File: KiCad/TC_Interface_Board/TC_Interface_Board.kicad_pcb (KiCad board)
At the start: 2 copper layers, 30 parts, among them J10 Conn_01x05, J11 Conn_01x05, J1_24V_ROW1 Conn_01x04, J1_CN1_24V1 Conn_01x03, J2_CN2_9V_Main1 Conn_01x02, J3_CN3_9V_Main1 Conn_01x02, J4 Conn_01x05, J5 Conn_01x05, J6 Conn_01x05, J7 Conn_01x05, J8 Conn_01x05, J9 Conn_01x05, Q1 DTC143E, Q2 DTC143E, U1 MC34063AP

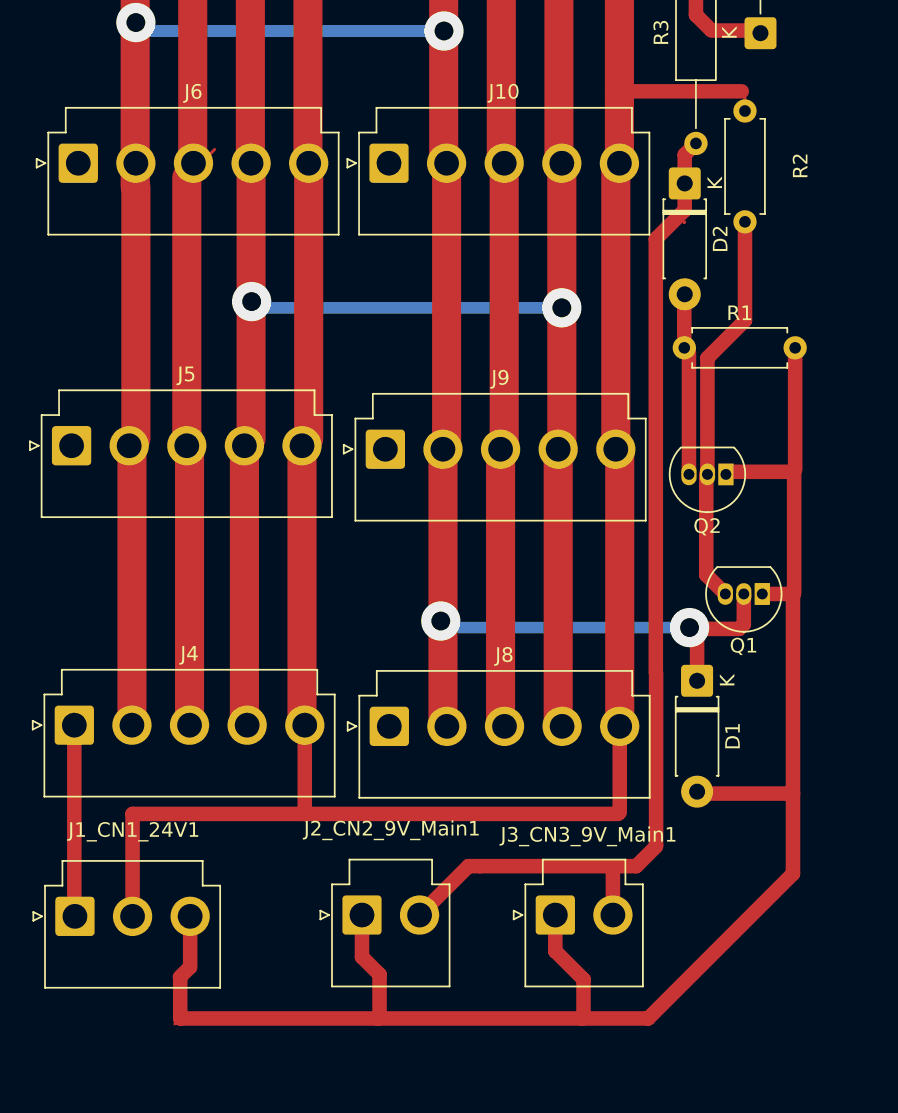
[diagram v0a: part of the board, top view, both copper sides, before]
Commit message: UPDATE
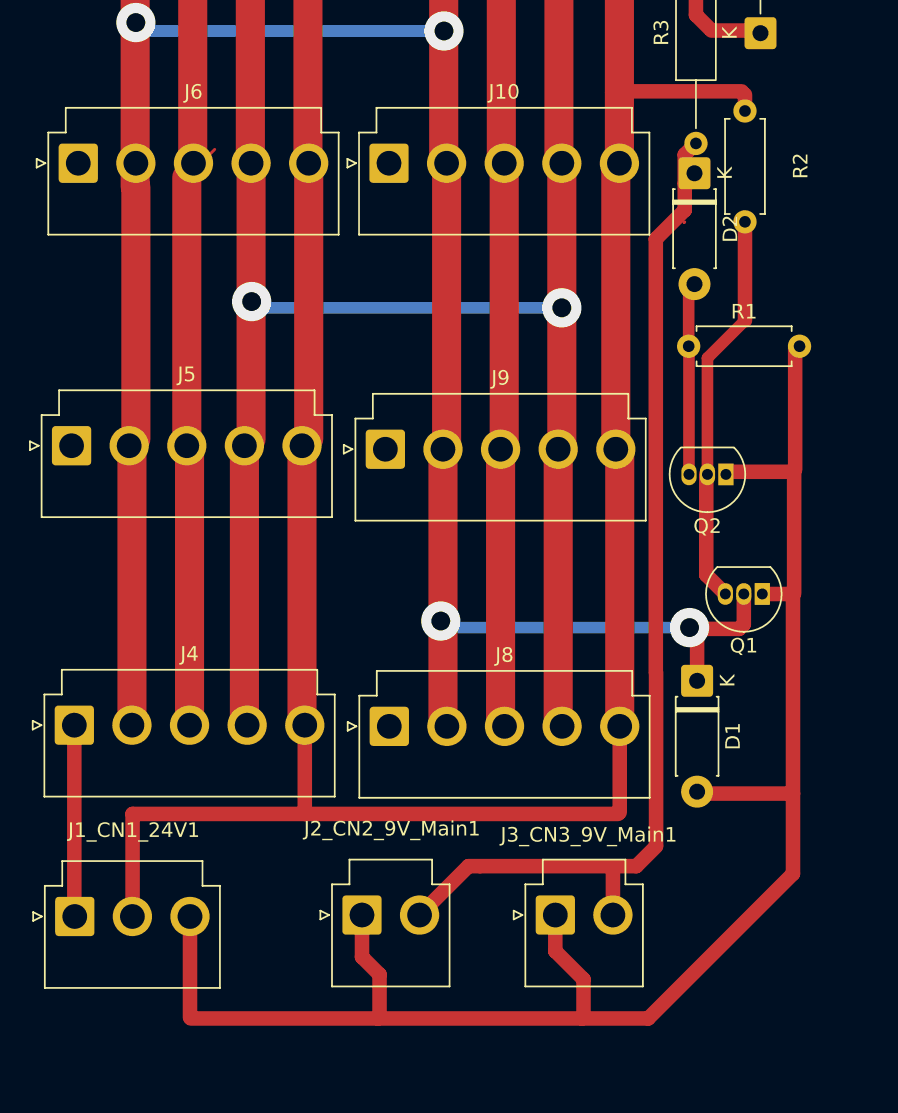
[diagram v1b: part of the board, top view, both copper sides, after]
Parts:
- moved D2 0.97 mm to (166.3, 89.9)
- moved R1 0.32 mm to (165.9, 101.8)
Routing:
- net Net-(D1-A): track 121.5 -> 119.9 mm
- net Net-(D2-A): track 12.5 -> 13.3 mm
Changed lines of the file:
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@@
 	(footprint "Resistor_THT:R_Axial_DIN0207_L6.3mm_D2.5mm_P7.62mm_Horizontal"
 		(layer "F.Cu")
-		(at 165.64 101.92)
+		(at 165.94 101.81)
 		(descr "Resistor, Axial_DIN0207 series, Axial, Horizontal, pin pitch=7.62mm, 0.25W = 1/4W, length*diameter=6.3*2.5mm^2, http://cdn-reichelt.de/documents/datenblatt/B400/1_4W%23YAG.pdf")
 		(tags "Resistor Axial_DIN0207 series Axial Horizontal pin pitch 7.62mm 0.25W = 1/4W length 6.3mm diameter 2.5mm")
@@
 	(footprint "Diode_THT:D_DO-41_SOD81_P7.62mm_Horizontal"
 		(layer "F.Cu")
-		(at 165.67 90.62 -90)
+		(at 166.34 89.92 -90)
 		(descr "Diode, DO-41_SOD81 series, Axial, Horizontal, pin pitch=7.62mm, length*diameter=5.2*2.7mm^2, https://www.diodes.com/assets/Package-Files/DO-41-Plastic.pdf")
 		(tags "Diode DO-41_SOD81 series Axial Horizontal pin pitch 7.62mm  length 5.2mm diameter 2.7mm")
@@
 	(footprint "Connector_JST:JST_VH_B3P-VH-B_1x03_P3.96mm_Vertical"
 		(layer "F.Cu")
-		(at 123.7525 141)
+		(at 123.74 141.01)
 		(descr "JST VH PBT series connector, B3P-VH-B (http://www.jst-mfg.com/product/pdf/eng/eVH.pdf), generated with kicad-footprint-generator")
 		(tags "connector JST VH vertical")
@@
 		(start 165.96 110.62)
 		(end 165.96 102.24)
-		(width 1)
+		(width 0.8)
 		(layer "F.Cu")
 		(net 2)
 	)
 	(segment
-		(start 165.64 101.92)
-		(end 165.64 98.27)
-		(width 1)
+		(start 165.94 97.94)
+		(end 166.34 97.54)
+		(width 0.2)
 		(layer "F.Cu")
 		(net 2)
@@
 	)
 	(segment
+		(start 165.94 101.81)
+		(end 165.94 97.94)
+		(width 0.8)
+		(layer "F.Cu")
+		(net 2)
+	)
+	(segment
 		(start 162.43 58.71)
 		(end 162.43 60.646428)
@@
 	)
 	(segment
-		(start 130.966428 145.18)
-		(end 131.626428 144.52)
-		(width 1)
-		(layer "F.Cu")
-		(net 8)
-	)
-	(segment
 		(start 168.68 110.44)
 		(end 168.5 110.62)
@@
 	)
 	(segment
-		(start 130.99 148.02)
-		(end 144.58 148.02)
-		(width 1)
-		(layer "F.Cu")
-		(net 8)
-	)
-	(segment
 		(start 173.16 118.84)
 		(end 173.19 118.81)
@@
 	)
 	(segment
-		(start 131.656428 144.52)
-		(end 131.6725 144.503928)
-		(width 0.2)
-		(layer "F.Cu")
-		(net 8)
-	)
-	(segment
 		(start 158.71 145.33)
 		(end 158.71 147.91)
@@
 	)
 	(segment
+		(start 131.72 148.02)
+		(end 144.58 148.02)
+		(width 1)
+		(layer "F.Cu")
+		(net 8)
+	)
+	(segment
 		(start 144.58 148.02)
 		(end 158.6 148.02)
@@
 	)
 	(segment
-		(start 130.99 145.203572)
-		(end 130.966428 145.18)
-		(width 0.2)
+		(start 173.11 132.56)
+		(end 173.11 118.96)
+		(width 1)
 		(layer "F.Cu")
 		(net 8)
 	)
 	(segment
-		(start 173.11 132.56)
-		(end 173.11 118.96)
-		(width 1)
+		(start 131.72 148.02)
+		(end 131.66 147.96)
+		(width 0.2)
 		(layer "F.Cu")
 		(net 8)
@@
 	)
 	(segment
-		(start 131.6725 144.503928)
-		(end 131.6725 141)
-		(width 1)
-		(layer "F.Cu")
-		(net 8)
-	)
-	(segment
 		(start 173.26 110.29)
 		(end 173.26 101.92)
@@
 	)
 	(segment
-		(start 131.626428 144.52)
-		(end 131.656428 144.52)
-		(width 0.2)
-		(layer "F.Cu")
-		(net 8)
-	)
-	(segment
 		(start 143.4825 143.7925)
 		(end 144.69 145)
@@
 	)
 	(segment
-		(start 130.61 148.4)
-		(end 130.99 148.02)
-		(width 0.2)
+		(start 131.66 147.96)
+		(end 131.66 141.01)
+		(width 1)
 		(layer "F.Cu")
 		(net 8)
@@
 	)
 	(segment
-		(start 130.99 148.02)
-		(end 130.99 145.203572)
-		(width 1)
-		(layer "F.Cu")
-		(net 8)
-	)
-	(segment
 		(start 167.15 117.53)
 		(end 167.15 110.62)
@@
 		(start 167.23 102.62)
 		(end 169.81 100.04)
-		(width 1)
+		(width 0.8)
 		(layer "F.Cu")
 		(net 9)
@@
 		(start 167.23 110.62)
 		(end 167.23 102.62)
-		(width 1)
+		(width 0.8)
 		(layer "F.Cu")
 		(net 9)
@@
 		(start 169.81 85.64)
 		(end 169.81 84.51)
-		(width 0.2)
+		(width 1)
 		(layer "F.Cu")
 		(net 16)

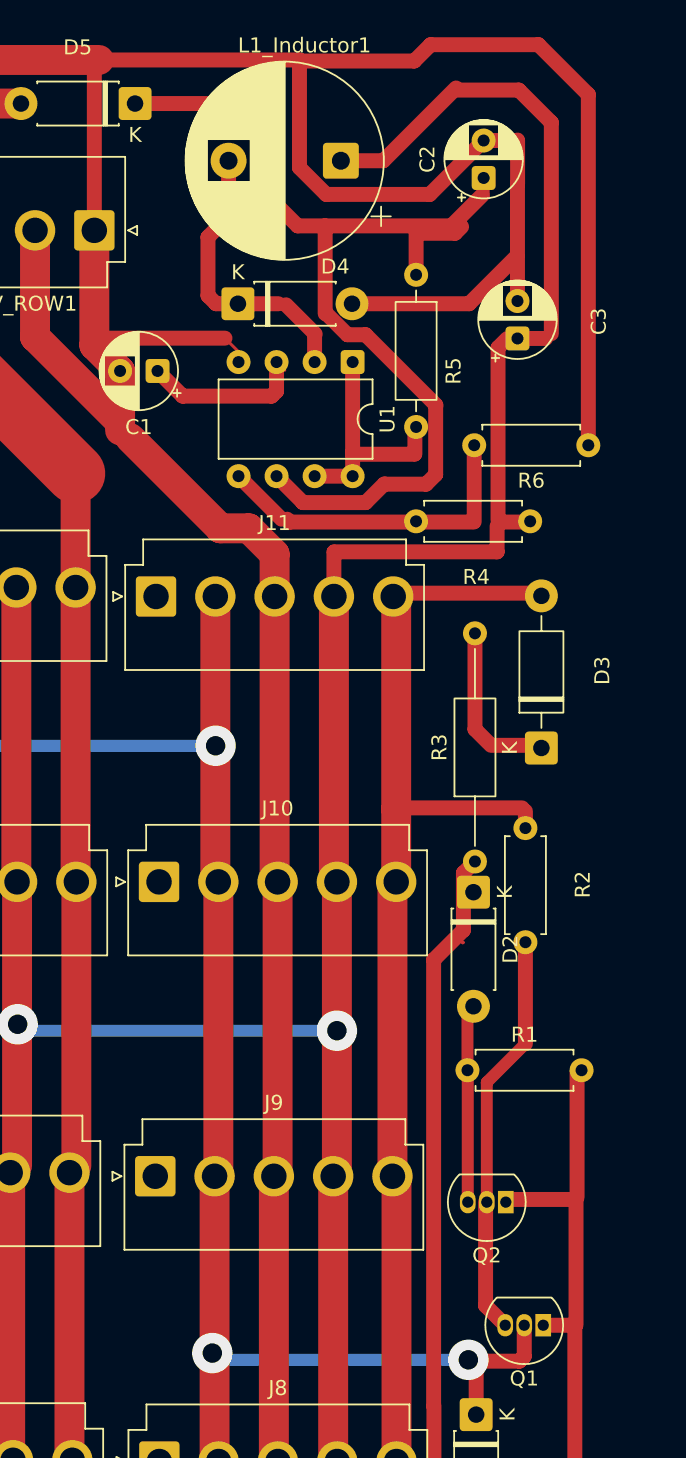
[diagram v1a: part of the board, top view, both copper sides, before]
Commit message: UPDATE
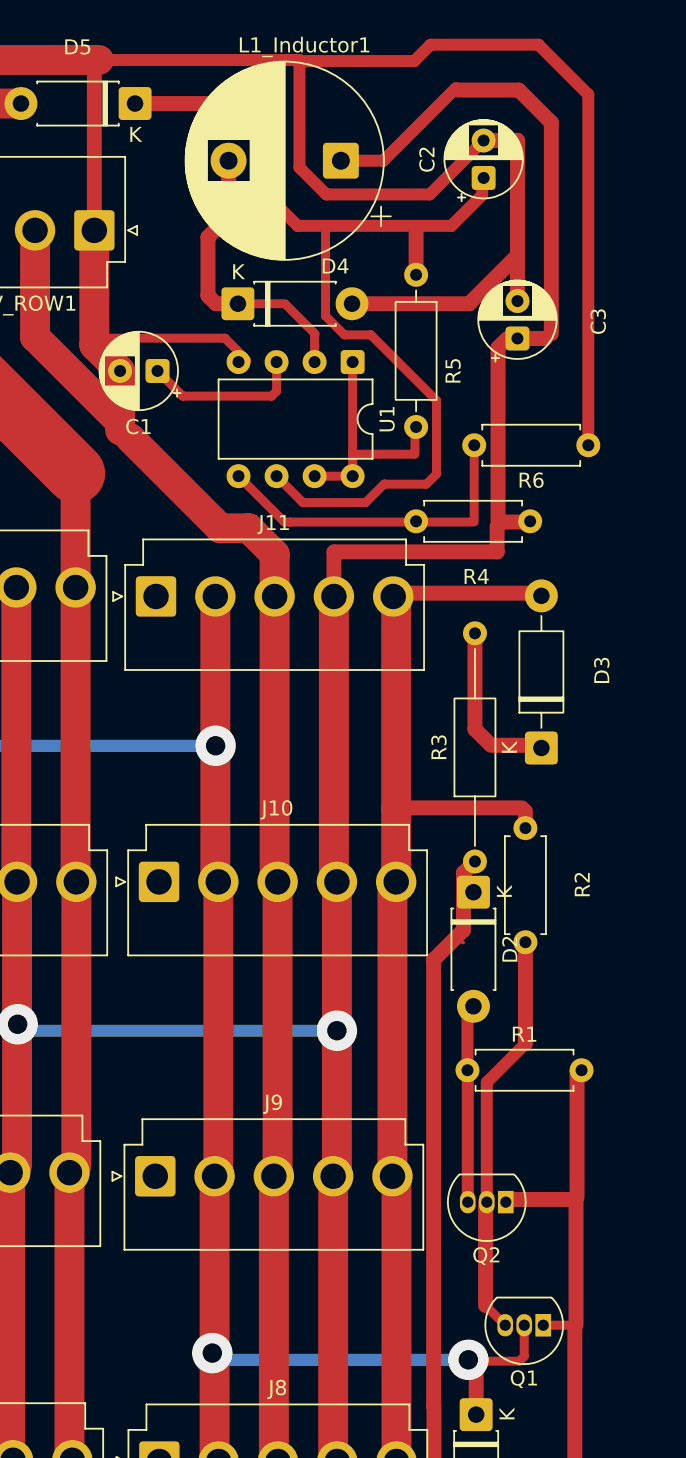
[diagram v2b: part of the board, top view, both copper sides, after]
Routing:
- net Net-(D5-K): track 73.3 -> 66.8 mm
